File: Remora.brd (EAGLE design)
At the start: 86.4 x 66.7 mm, 81 parts, among them IC1 MCP23017, J2 GROVE-I2C, P1 PADSMALL, T1 2N3904, T2 BSS138

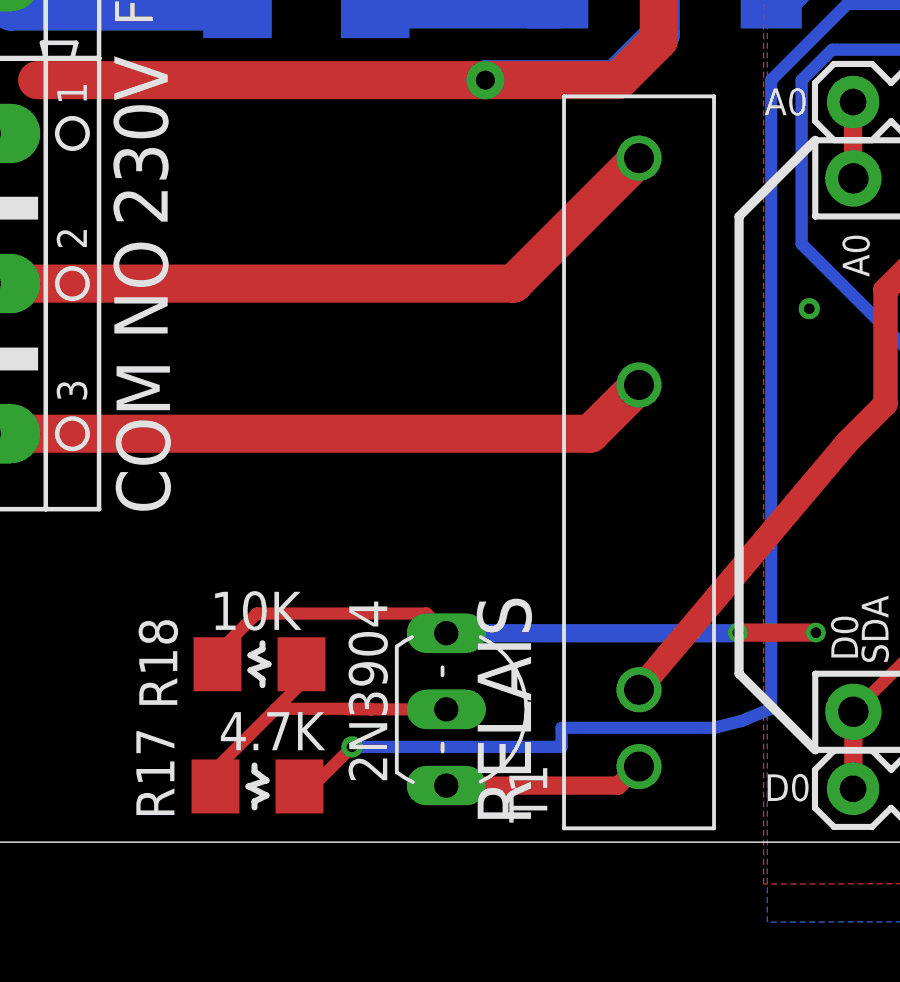
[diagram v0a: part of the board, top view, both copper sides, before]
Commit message: Mise à jour du PCB et ajout d'images
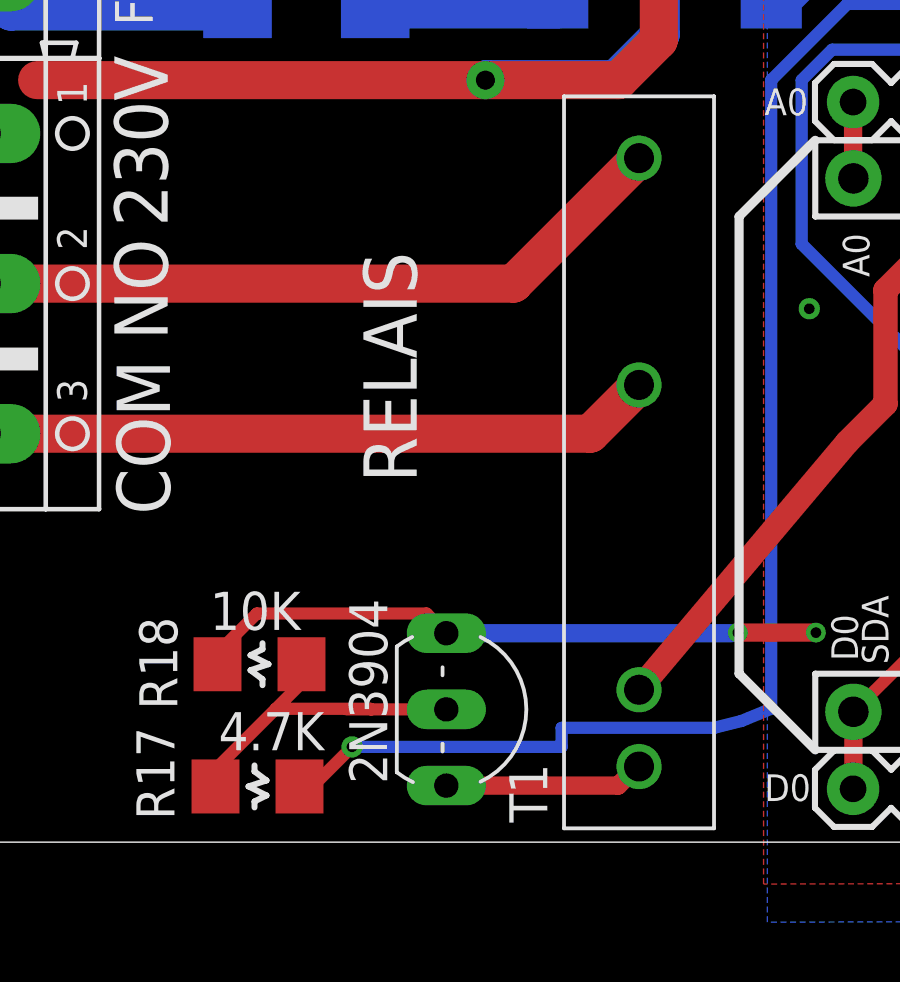
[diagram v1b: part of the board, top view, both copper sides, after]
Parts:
- RELAIS: value G3MC-202P -> G3MC-202P-5V
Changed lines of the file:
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@@
 <attribute name="OC_FARNELL" value="unknown" x="4.7752" y="18.6182" size="1.778" layer="27" rot="R270" display="off"/>
 </element>
-<element name="RELAIS" library="sip-4" package="SIP-4" value="G3MC-202P" x="26.67" y="12.7" rot="R90"/>
+<element name="RELAIS" library="sip-4" package="SIP-4" value="G3MC-202P-5V" x="26.67" y="12.7" smashed="yes" rot="R90">
+<attribute name="NAME" x="19.3" y="11.99" size="1.778" layer="25" rot="R90"/>
+<attribute name="VALUE" x="23.05" y="7.81" size="1.778" layer="27" rot="R90"/>
+</element>
 </elements>
 <signals>
